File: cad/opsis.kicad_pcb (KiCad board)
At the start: 2 copper layers, 100 x 70 mm, 18 parts, among them J101 Conn_01x02, J102 Conn_01x02, J103 Conn_01x02, J104 REGULATOR, J105 Conn_01x02, J106 Conn_01x02, J107 Conn_01x04_MountingPin, J108 Conn_01x02, J109 USB_A

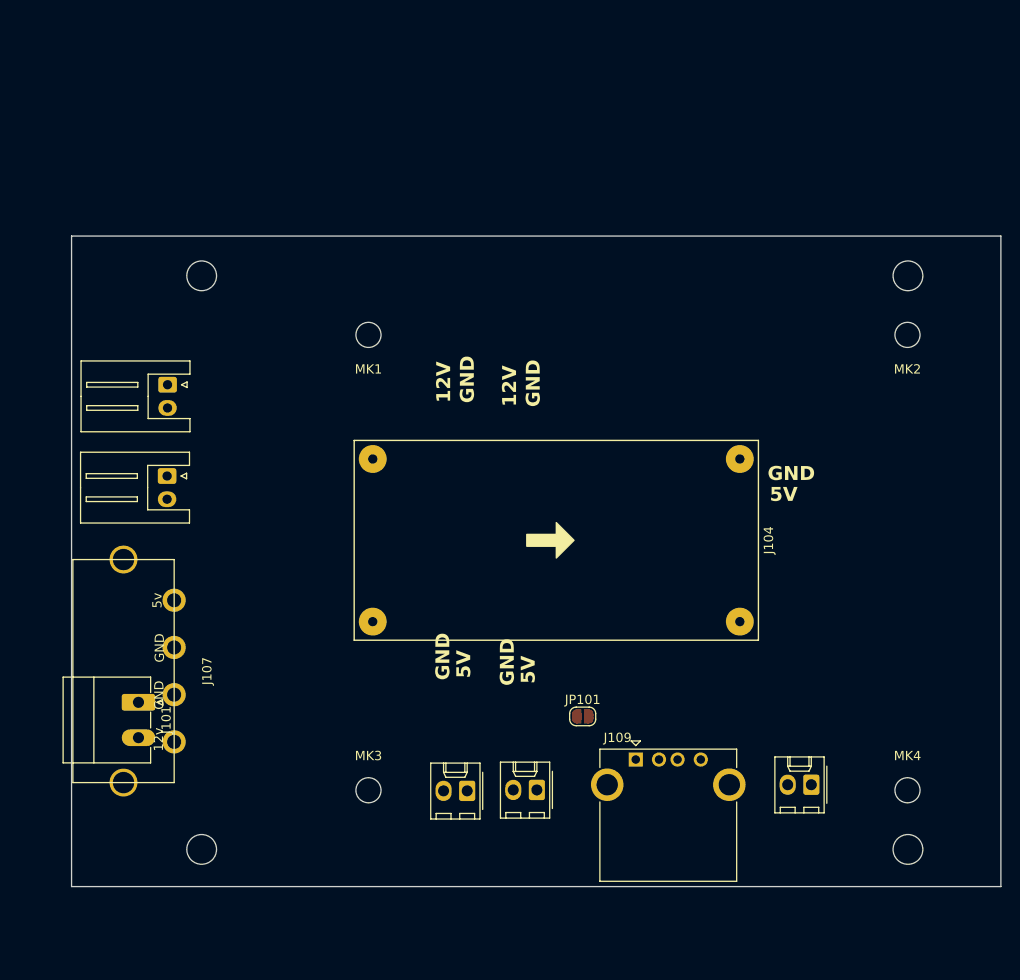
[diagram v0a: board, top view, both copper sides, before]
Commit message: initial rev made
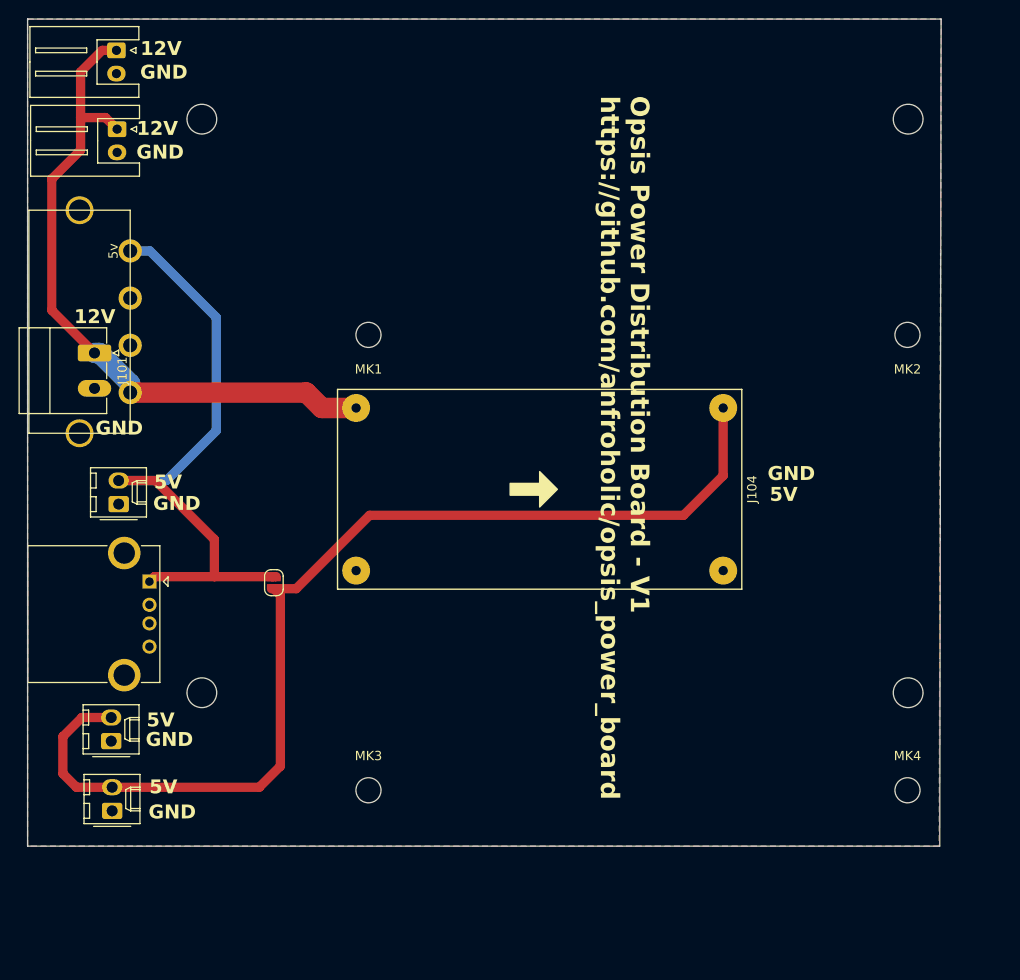
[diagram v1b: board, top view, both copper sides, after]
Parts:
- moved J108 80.4 mm to (33.8, 82.2), turned to 90 degrees
- moved J109 55.7 mm to (37.1, 90.5), turned to -90 degrees
- moved J107 45.8 mm to (33.1, 115.2), turned to 90 degrees
- moved J106 38.7 mm to (33.0, 107.7), turned to 90 degrees
- moved J105 37.9 mm to (29.6, 62.6)
- moved J101 37.9 mm to (31.2, 65.9)
- moved J102 37.7 mm to (33.6, 41.9)
- moved J103 36.4 mm to (33.6, 33.4)
- moved JP101 36.2 mm to (50.5, 90.7), turned to 90 degrees
- moved H101 16.9 mm to (42.8, 40.8)
- moved H102 16.9 mm to (118.8, 40.8)
- moved H103 16.9 mm to (118.8, 102.5)
- moved H104 16.9 mm to (42.8, 102.5)
- moved J104 5.77 mm to (79.1, 80.6)
- renumbered J107 to J105, J105 to J106, J106 to J107
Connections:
- J105 pad MP: unconnected-(J107-MountPin-PadMP) -> GND
- J106 pad 1: Net-(J104-Pin_4) -> GND
- J106 pad 2: GND -> Net-(J104-Pin_4)
- J107 pad 1: Net-(J104-Pin_4) -> GND
- J107 pad 2: GND -> Net-(J104-Pin_4)
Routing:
- net Net-(J104-Pin_4): track 0.00 -> 115.0 mm
- net Net-(J101-Pin_1): track 0.00 -> 73.9 mm
- net Net-(J105-Pin_4): track 0.00 -> 67.7 mm
- added copper zone on B.Cu, net GND
- added copper zone on F.Cu, net GND
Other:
- board size 100 x 70 mm -> 98.3 x 89 mm
- board text added: "Opsis Power Distribution Board - V1 https://github.com/anfroholic/opsis_power_board"
